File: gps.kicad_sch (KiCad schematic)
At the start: 16 parts, among them U2 GY-NEO6MV2, U3 24AA32AT-I_SN

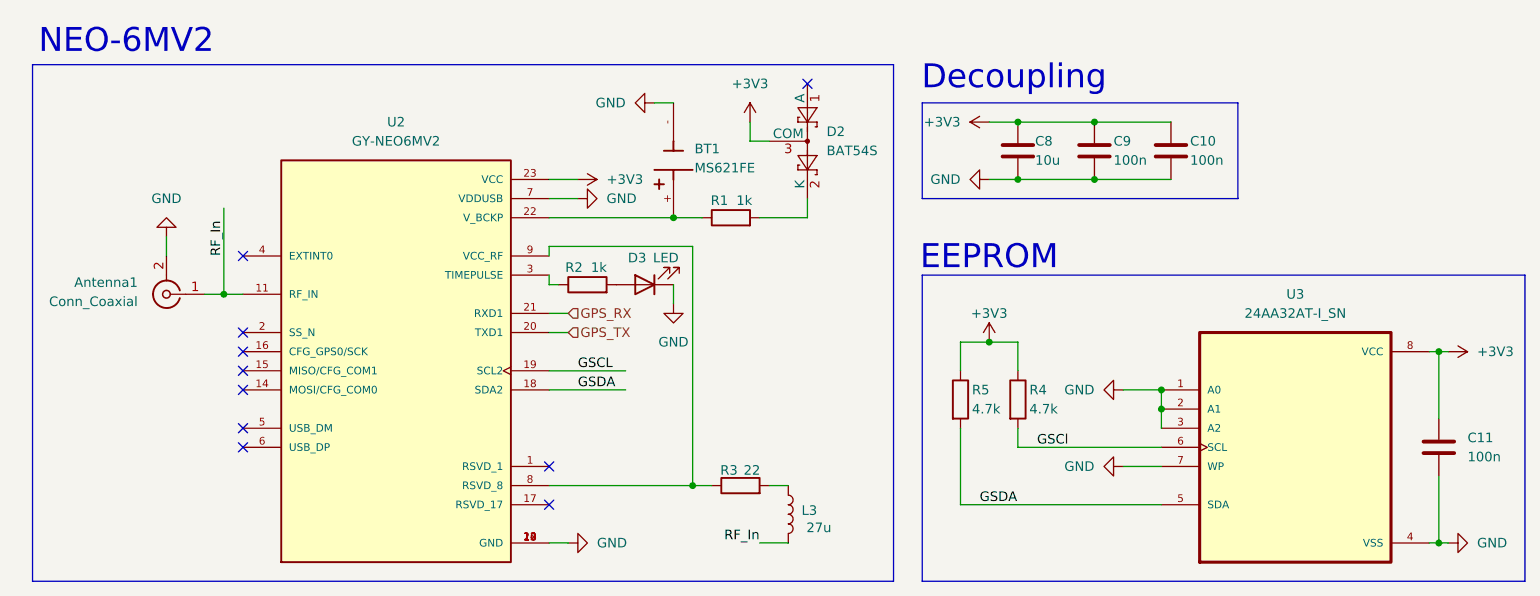
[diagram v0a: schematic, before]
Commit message: Sensors & Main board start
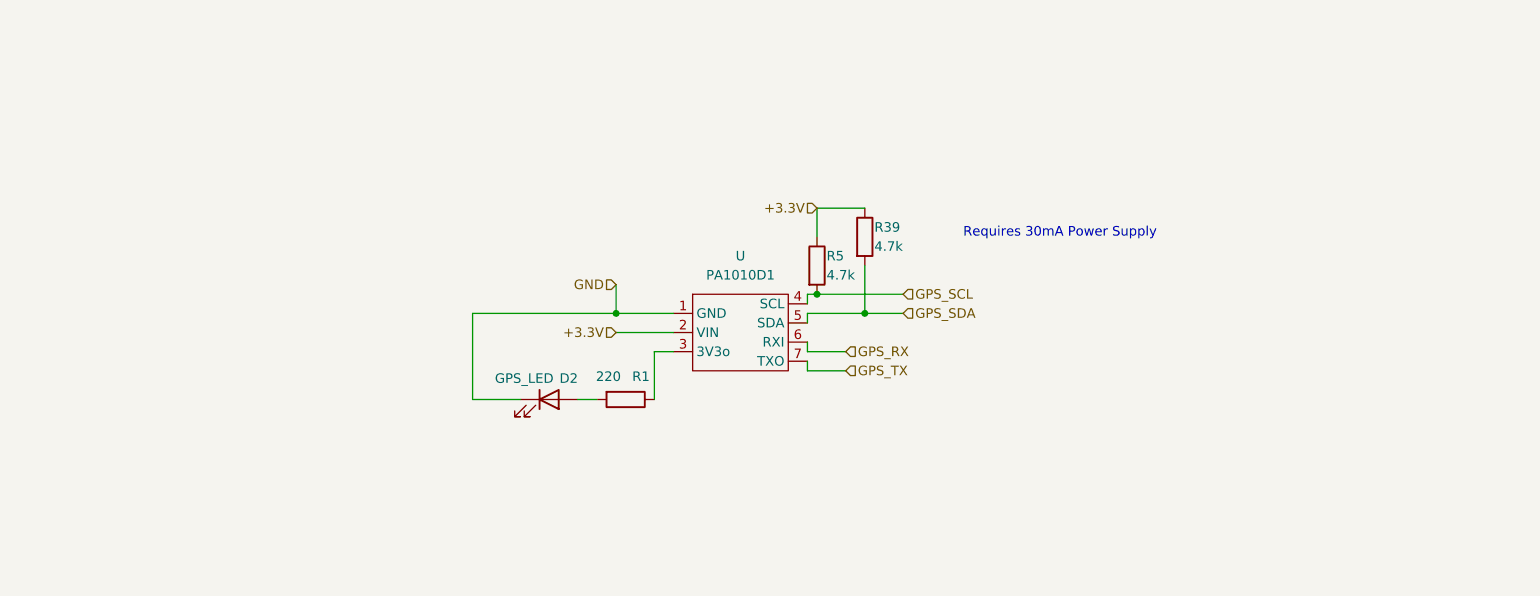
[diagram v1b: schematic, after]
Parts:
- removed Antenna1: Conn_Coaxial, Connector_Coaxial:U.FL_Hirose_U.FL-R-SMT-1_Vertical, symbol Connector:Conn_Coaxial
- removed BT1: MS621FE, MS621FE-FL11E:BAT_MS621FE-FL11E, symbol MS621FE-FL11E:MS621FE-FL11E
- removed C10, C11, C9: 100n, symbol Device:C
- removed C8: 10u, symbol Device:C
- removed D2: BAT54S, Package_TO_SOT_SMD:SOT-23, symbol Diode:BAT54S
- removed D3: LED, symbol Device:LED
- removed L3: 27u, symbol Device:L
- removed R2: 1k, symbol Device:R
- removed R3: 22, symbol Device:R
- removed R4: 4.7k, symbol Device:R
- removed U2: GY-NEO6MV2, GY-NEO6MV2:XCVR_GY-NEO6MV2, symbol GY-NEO6MV2:GY-NEO6MV2
- removed U3: 24AA32AT-I_SN, 24AA32AT-I_SN:SOIC127P600X175-8N, symbol 24AA32AT-I_SN:24AA32AT-I_SN
- added D2: GPS_LED, symbol Device:LED
- added R39: 4.7k, symbol Device:R
- added U: PA1010D1, symbol CustomFPs:Adafruit_Mini_GPS_PA1010D
- R1: value 1k -> 220
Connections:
- net GND: now also D2.1 (K), U.1 (GND)
- net GPS_RX: now also U.6 (RXI)
- net GPS_TX: now also U.7 (TXO)
- net at R1.1: now also U.3 (3V3o)
- net at R1.2: now also D2.2 (A)
- net +3V3 renamed +3.3V
- net +3.3V: now also R39.1, U.2 (VIN)
- net GSDA renamed GPS_SCL
- net GPS_SCL: now also U.4 (SCL)
- new net GPS_SDA: R39.2, U.5 (SDA)
- no-connect marks 10 -> 0
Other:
- note added: "Requires 30mA Power Supply"
- note removed: "Decoupling"
- note removed: "EEPROM"
- note removed: "NEO-6MV2"
